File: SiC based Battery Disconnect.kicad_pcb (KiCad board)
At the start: 4 copper layers, 111 x 74.6 mm, 93 parts, among them IC2 PIC16F15345T-E_SSVAO, IC4 MCP1792T-5002H_CB, IC5 MCP1792T-5002H_CB, J1 Input, J2 Output, J3 12V supply, J5 490107670612, J6 490107670612, Q1 IMW120R014M1H, Q2 IMW120R014M1H, Q3 2N7002BK,215, Q4 Si2333DS, Q5 2N7002BK,215, Q6 2N7002bk,215, T1 760390014, U1 PIC10F322-IOT, U2 MCP6022, U4 TC4432VOA

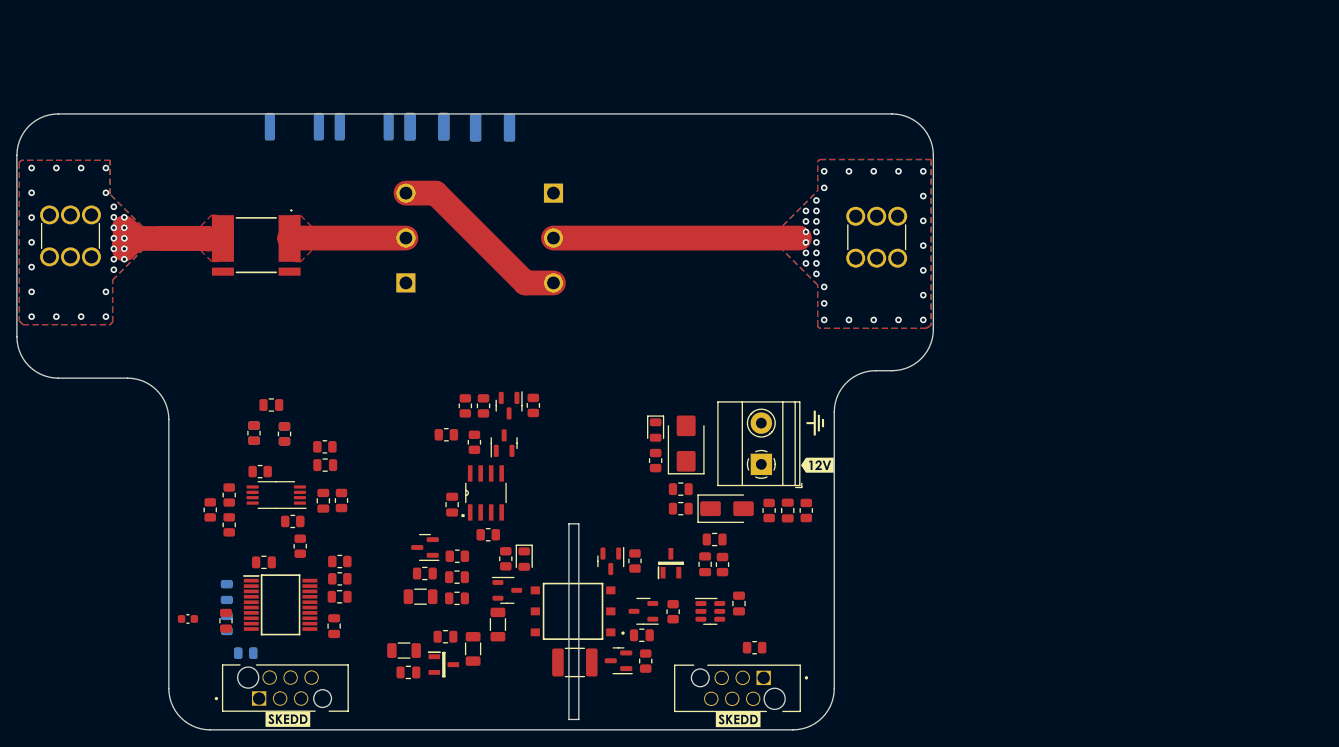
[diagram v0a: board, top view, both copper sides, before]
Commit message: updated the design
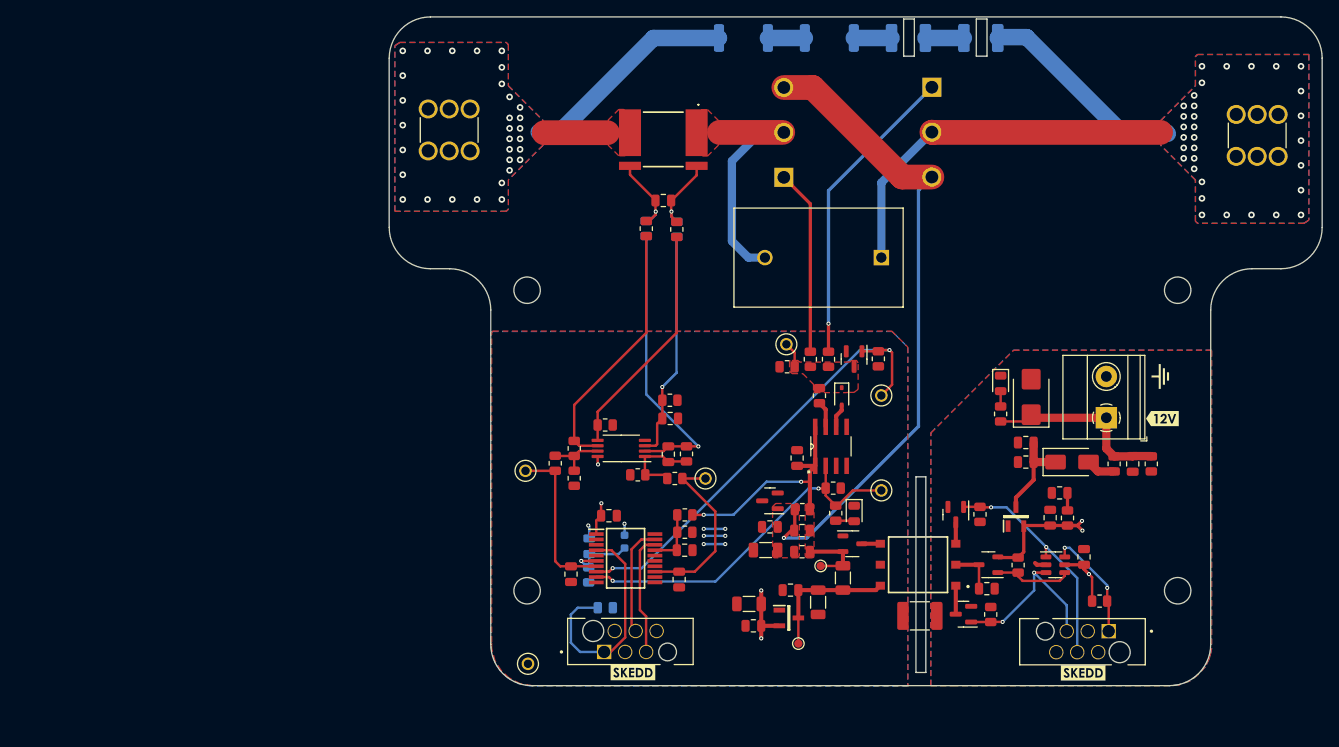
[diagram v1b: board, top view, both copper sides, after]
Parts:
- added H1: MountingHole, MountingHole:MountingHole_3.2mm_M3, F.Cu at (193.8, 137.3)
- added H2: MountingHole, MountingHole:MountingHole_3.2mm_M3, F.Cu at (115.0, 137.3)
- added H3: MountingHole, MountingHole:MountingHole_3.2mm_M3, F.Cu at (193.8, 100.9)
- added H4: MountingHole, MountingHole:MountingHole_3.2mm_M3, F.Cu at (115.0, 100.9)
- added RV1: Varistor, Varistor:VARRB750W100L2050T1200H2800, F.Cu at (150.3, 96.9)
- added TP1: 5001, 5001 tp:KEYSTONE_5001, F.Cu at (157.9, 125.1)
- added TP2: 5001, 5001 tp:KEYSTONE_5001, F.Cu at (157.9, 113.6)
- added TP3: TestPoint, TestPoint:TestPoint_Pad_D1.0mm, F.Cu at (147.9, 143.7)
- added TP5: 5001, 5001 tp:KEYSTONE_5001, F.Cu at (115.1, 146.1)
- added TP6: 5001, 5001 tp:KEYSTONE_5001, F.Cu at (136.6, 123.7)
- added TP7: 5001, 5001 tp:KEYSTONE_5001, F.Cu at (114.8, 122.8)
- added TP8: TestPoint, TestPoint:TestPoint_Pad_D1.0mm, F.Cu at (150.6, 134.3)
- added TP9: 5001, 5001 tp:KEYSTONE_5001, F.Cu at (146.4, 107.4)
- D7: value BZX84J-B22,115_22V -> BZX384-B22,115; footprint Package_TO_SOT_SMD:SOT-23 -> Diode_SMD:D_SOD-323
- Q6: value 2N7002bk,215 -> 2N7002BK,215
- TH100: moved to B.Cu
- moved C16 60.1 mm to (170.0, 70.3)
- moved C17 59.3 mm to (161.2, 70.3)
- moved R26 57.4 mm to (151.6, 70.3)
- moved R27 55.5 mm to (141.2, 70.3)
- moved TH100 53.7 mm to (126.8, 131.3), turned to 90 degrees
- moved R17 53.6 mm to (129.4, 93.4)
- moved R16 53.6 mm to (133.1, 93.5)
- moved R15 53.6 mm to (129.4, 93.4)
- moved R14 53.6 mm to (133.1, 93.5)
- moved C15 53.6 mm to (131.5, 90.0)
- moved R3 50.9 mm to (131.5, 82.6)
- moved J1 47.7 mm to (200.9, 84.7)
- moved J2 47.6 mm to (103.0, 84.0)
- moved Q1 47.6 mm to (164.0, 76.3)
- moved Q2 47.5 mm to (146.1, 87.2)
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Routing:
- net VSOURCE: track 22.4 -> 79.2 mm, vias 0 -> 1
- net DRIVER_EN2: track 0.00 -> 56.2 mm, vias 0 -> 2
- net DRIVER_EN1: track 0.00 -> 44.3 mm, vias 0 -> 2
- net Net-(Q1-D): track 29.8 -> 70.9 mm
- net Net-(Q1-G): track 0.00 -> 37.6 mm, vias 0 -> 1
- net VCC: track 0.00 -> 36.9 mm, vias 0 -> 2
- net Net-(U2A--): track 0.00 -> 34.8 mm, vias 0 -> 1
- net Net-(U2B--): track 0.00 -> 31.5 mm
- net Net-(U2B-+): track 0.00 -> 28.6 mm
- net RA3: track 0.00 -> 27.9 mm
- net Net-(U2A-+): track 0.00 -> 27.7 mm, vias 0 -> 1
- net Net-(Q3-G): track 0.00 -> 27.5 mm, vias 0 -> 2
- net VDDLV: track 0.00 -> 23.1 mm, vias 0 -> 3
- net BATT+(12V-48V): track 0.00 -> 22.9 mm
- net Net-(Q2-G): track 0.00 -> 22.5 mm
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- added copper zone on F.Cu, net Earth
- added copper zone on F.Cu, net GND
- added copper zone on F.Cu, net Net-(D7-K)
- added copper zone on F.Cu, net VCC
- added copper zone on B.Cu, net VDDHV
- added copper zone on B.Cu, net VDDLV
- added copper zone on F.Cu, net VSOURCE
- removed copper zone on In1.Cu, net Net-(J2-Pad1)
- removed copper zone on In2.Cu, net Net-(J2-Pad1)
- removed copper zone on In1.Cu, net Net-(Q1-D)
- removed copper zone on In2.Cu, net Net-(Q1-D)
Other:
- board size 111 x 74.6 mm -> 113 x 81 mm
- copper layers 4 -> 2
